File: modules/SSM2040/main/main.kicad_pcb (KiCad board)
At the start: 2 copper layers, 40.3 x 111.8 mm, 60 parts, among them IC1 RC4136, J1 IDC Header, J2 Conn_01x07_Female, Q1 2N3906, U1 LM741, U2 SSM2040, U3 CA3080

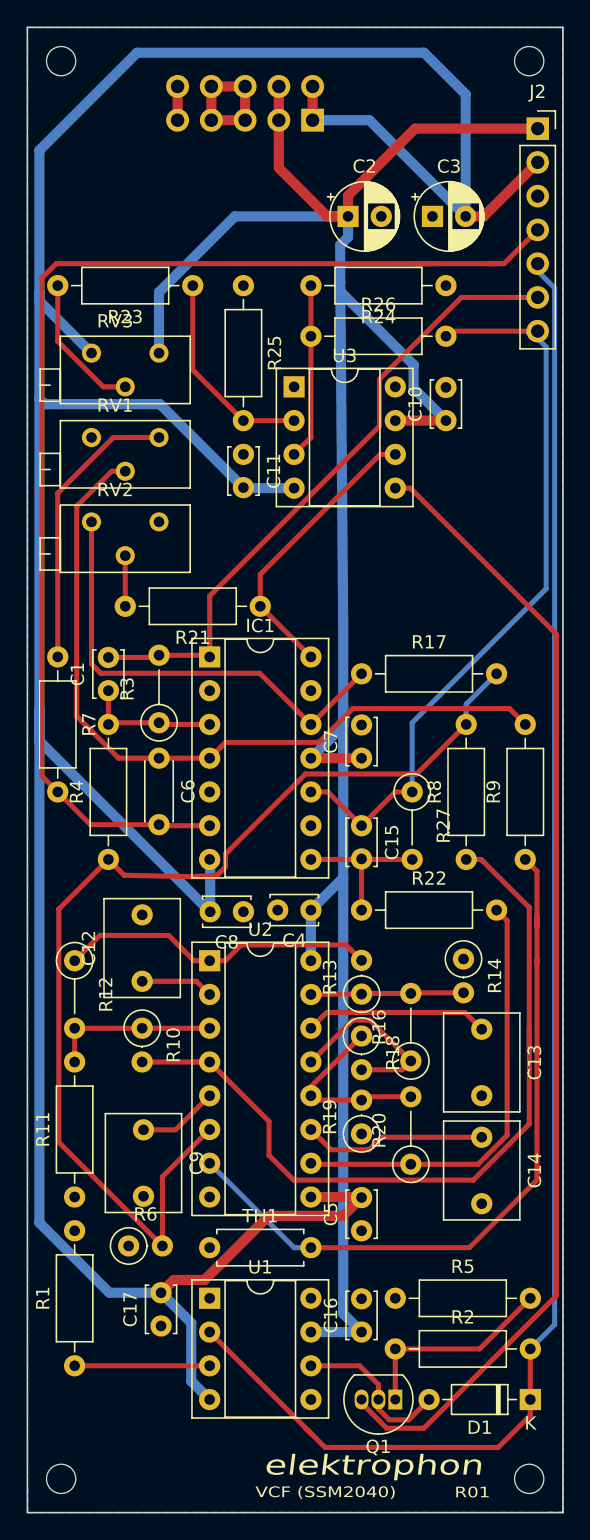
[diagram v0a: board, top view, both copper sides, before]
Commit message: finalize
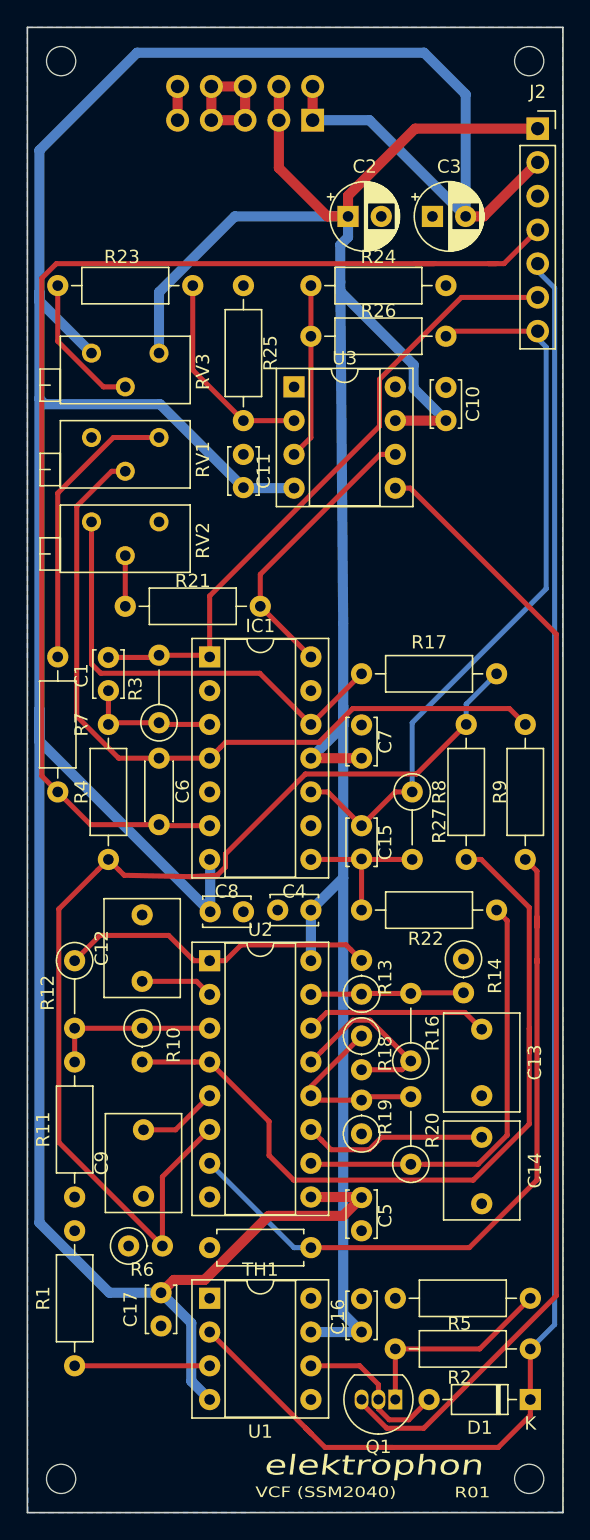
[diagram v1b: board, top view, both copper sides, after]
